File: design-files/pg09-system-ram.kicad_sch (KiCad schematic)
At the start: 14 parts, among them U601 74AHC139, U602 AS6C6264-55PCN, U603 AS6C4008-55PCN, U604 AS6C4008-55PCN, U605 AS6C4008-55PCN, U606 AS6C4008-55PCN, U607 AS6C4008-55PCN

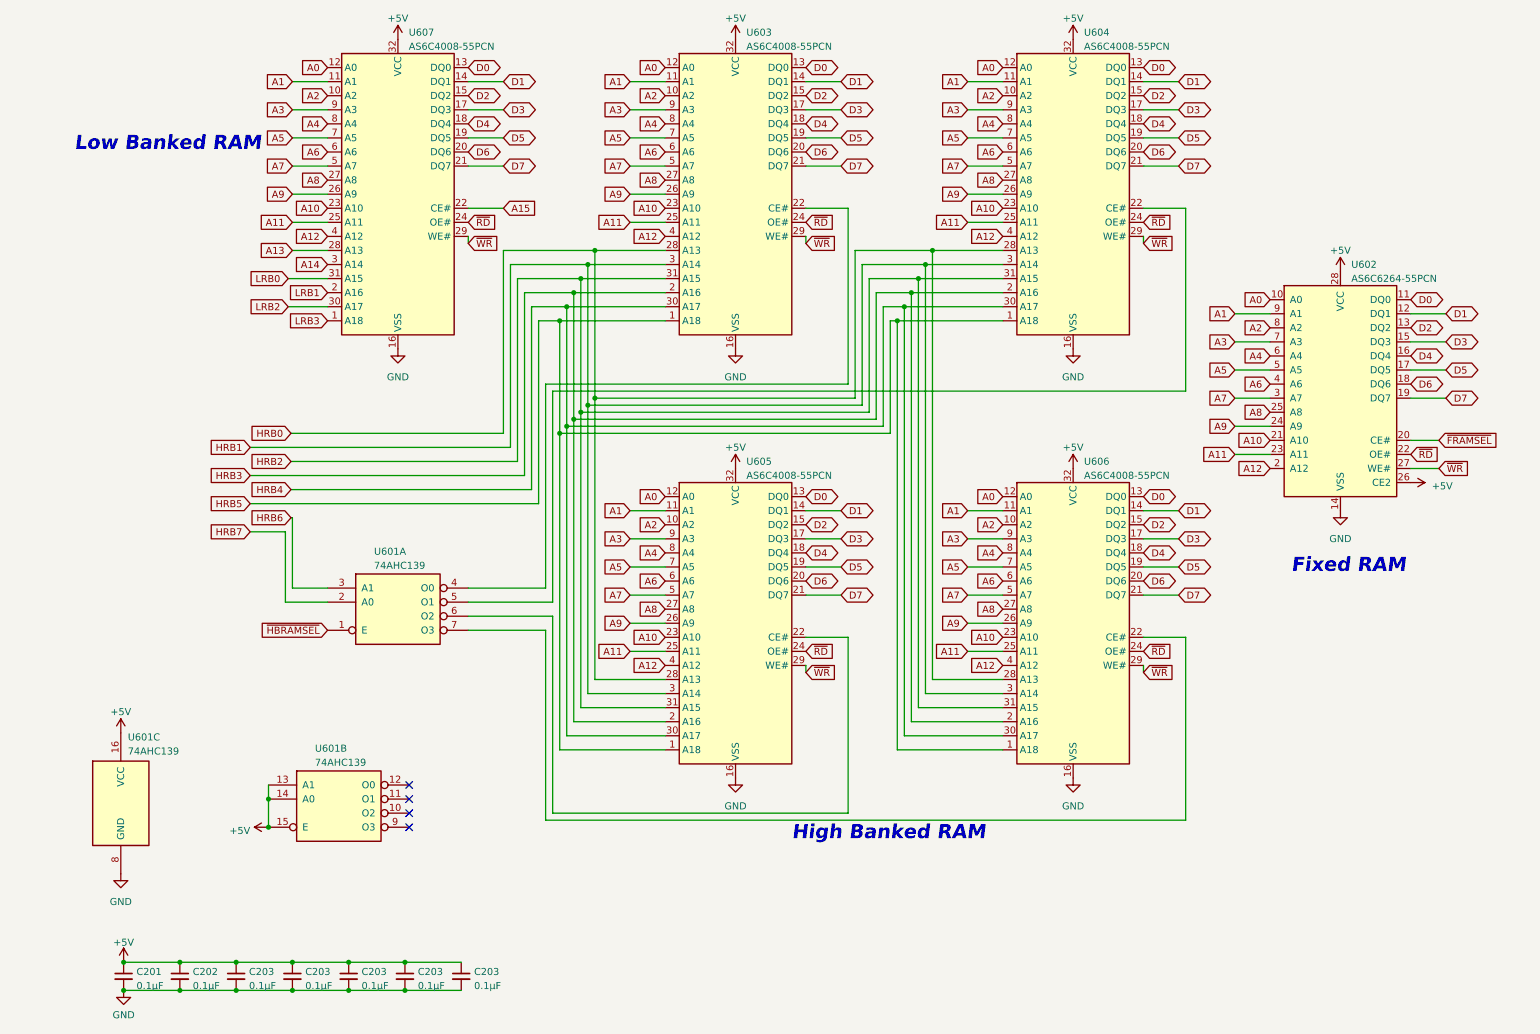
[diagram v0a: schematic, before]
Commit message: New banked RAM layout: - The 2MB RAM group is now Low Banked RAM, and divided into 2   16K independently bankable regions back by 1MB each. - The 512KB RAM is now High Banked RAM. - Shuffle the Low and High banker PIAs.
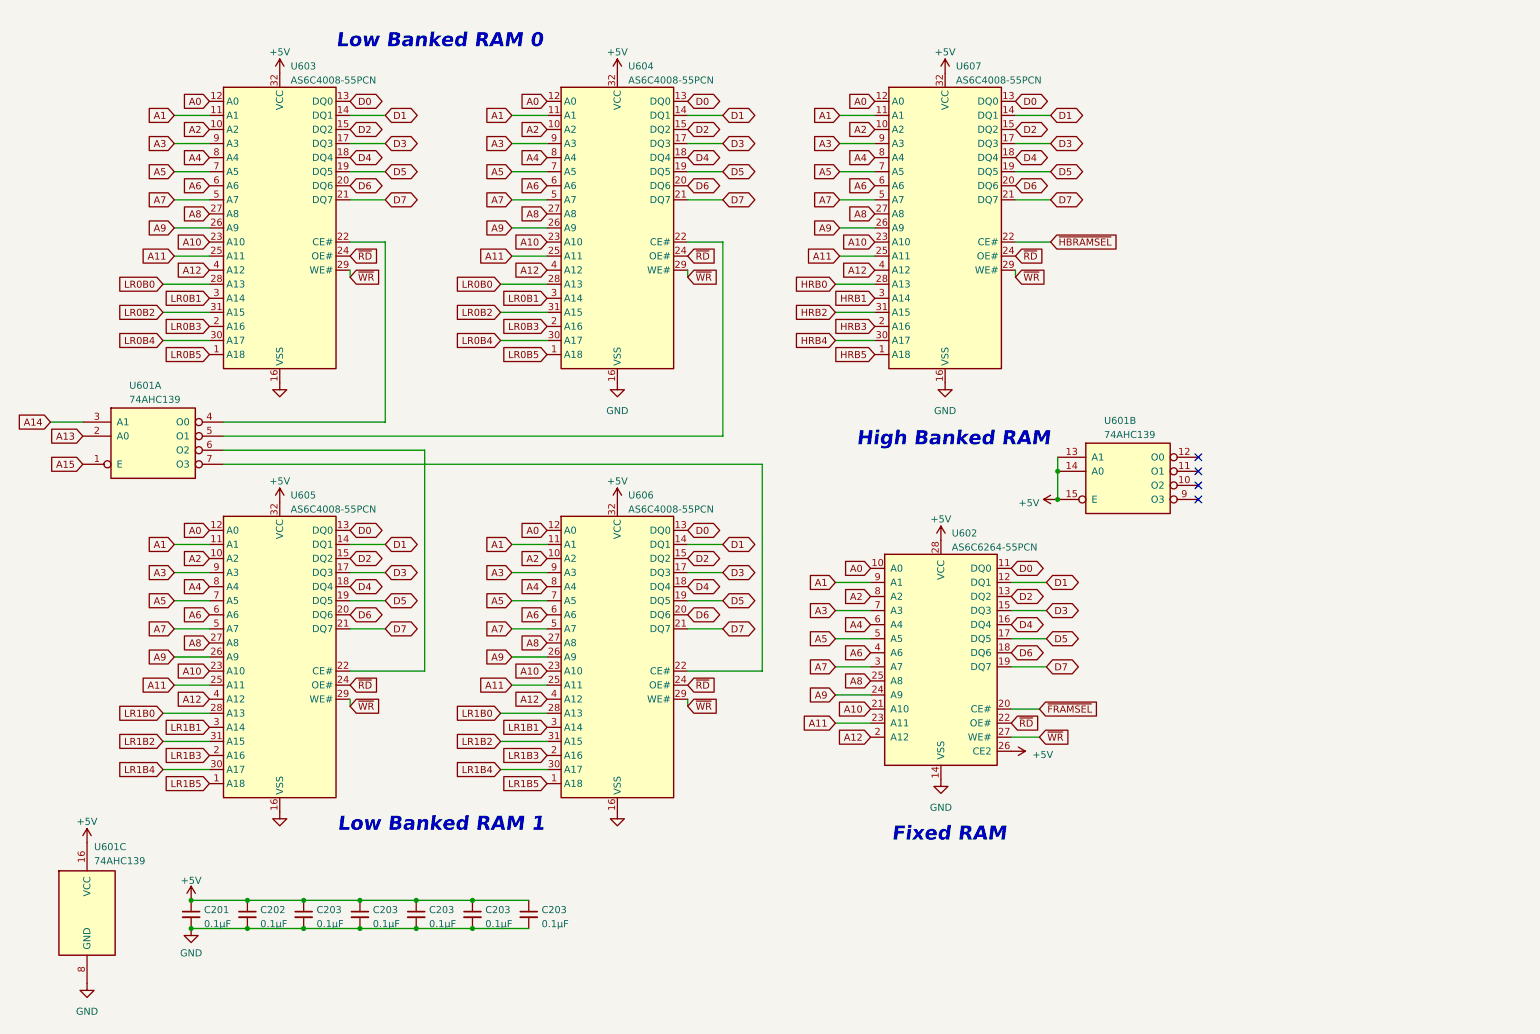
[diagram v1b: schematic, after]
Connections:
- net HRB6 is gone; now on net A14: U601.3 (A1)
- net HRB7 is gone; now on net A13: U601.2 (A0)
- net LRB0 is gone; now on net HRB2: U607.31 (A15)
- net LRB1 is gone; now on net HRB3: U607.2 (A16)
- net LRB2 is gone; now on net HRB4: U607.30 (A17)
- net LRB3 is gone; now on net HRB5: U607.1 (A18)
- net A13: no longer U607.28 (A13)
- net A14: no longer U607.3 (A14)
- net A15: now also U601.1 (E); no longer U607.22 (CE#)
- net HRB0: now also U607.28 (A13); no longer U603.28 (A13), U604.28 (A13), U605.28 (A13), U606.28 (A13)
- net HRB1: now also U607.3 (A14); no longer U603.3 (A14), U604.3 (A14), U605.3 (A14), U606.3 (A14)
- net HRB2: no longer U603.31 (A15), U604.31 (A15), U605.31 (A15), U606.31 (A15)
- net HRB3: no longer U603.2 (A16), U604.2 (A16), U605.2 (A16), U606.2 (A16)
- net HRB4: no longer U603.30 (A17), U604.30 (A17), U605.30 (A17), U606.30 (A17)
- net HRB5: no longer U603.1 (A18), U604.1 (A18), U605.1 (A18), U606.1 (A18)
- net ~{HBRAMSEL}: now also U607.22 (CE#); no longer U601.1 (E)
- new net LR0B0: U603.28 (A13), U604.28 (A13)
- new net LR0B1: U603.3 (A14), U604.3 (A14)
- new net LR0B2: U603.31 (A15), U604.31 (A15)
- new net LR0B3: U603.2 (A16), U604.2 (A16)
- new net LR0B4: U603.30 (A17), U604.30 (A17)
- new net LR0B5: U603.1 (A18), U604.1 (A18)
- new net LR1B0: U605.28 (A13), U606.28 (A13)
- new net LR1B1: U605.3 (A14), U606.3 (A14)
- new net LR1B2: U605.31 (A15), U606.31 (A15)
- new net LR1B3: U605.2 (A16), U606.2 (A16)
- new net LR1B4: U605.30 (A17), U606.30 (A17)
- new net LR1B5: U605.1 (A18), U606.1 (A18)
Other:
- note added: "Low Banked RAM 0"
- note added: "Low Banked RAM 1"
- note removed: "Low Banked RAM"
- moved on the sheet: C201, C202, C203, U601A, U601B, U601C, U602, U603, U604, U605, U606, U607
